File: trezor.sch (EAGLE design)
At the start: 38 parts, among them IC1 MCP1703CB, Q2 16MHz, U1 ATSHA204-TSU, U2 USB, U3 DISPLAY

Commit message: forgot to connect usb gnd/vcc
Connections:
- net +5V: now also U2.VBUS
- net GND: now also U2.GND
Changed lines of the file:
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@@
 <wire x1="99.06" y1="-20.32" x2="93.98" y2="-20.32" width="0.1524" layer="91"/>
 <wire x1="93.98" y1="-20.32" x2="93.98" y2="-25.4" width="0.1524" layer="91"/>
+<pinref part="U2" gate="G$1" pin="GND"/>
 </segment>
 </net>
@@
 <wire x1="109.22" y1="-22.86" x2="114.3" y2="-22.86" width="0.1524" layer="91"/>
 <wire x1="114.3" y1="-22.86" x2="114.3" y2="-20.32" width="0.1524" layer="91"/>
+<pinref part="U2" gate="G$1" pin="VBUS"/>
 </segment>
 </net>

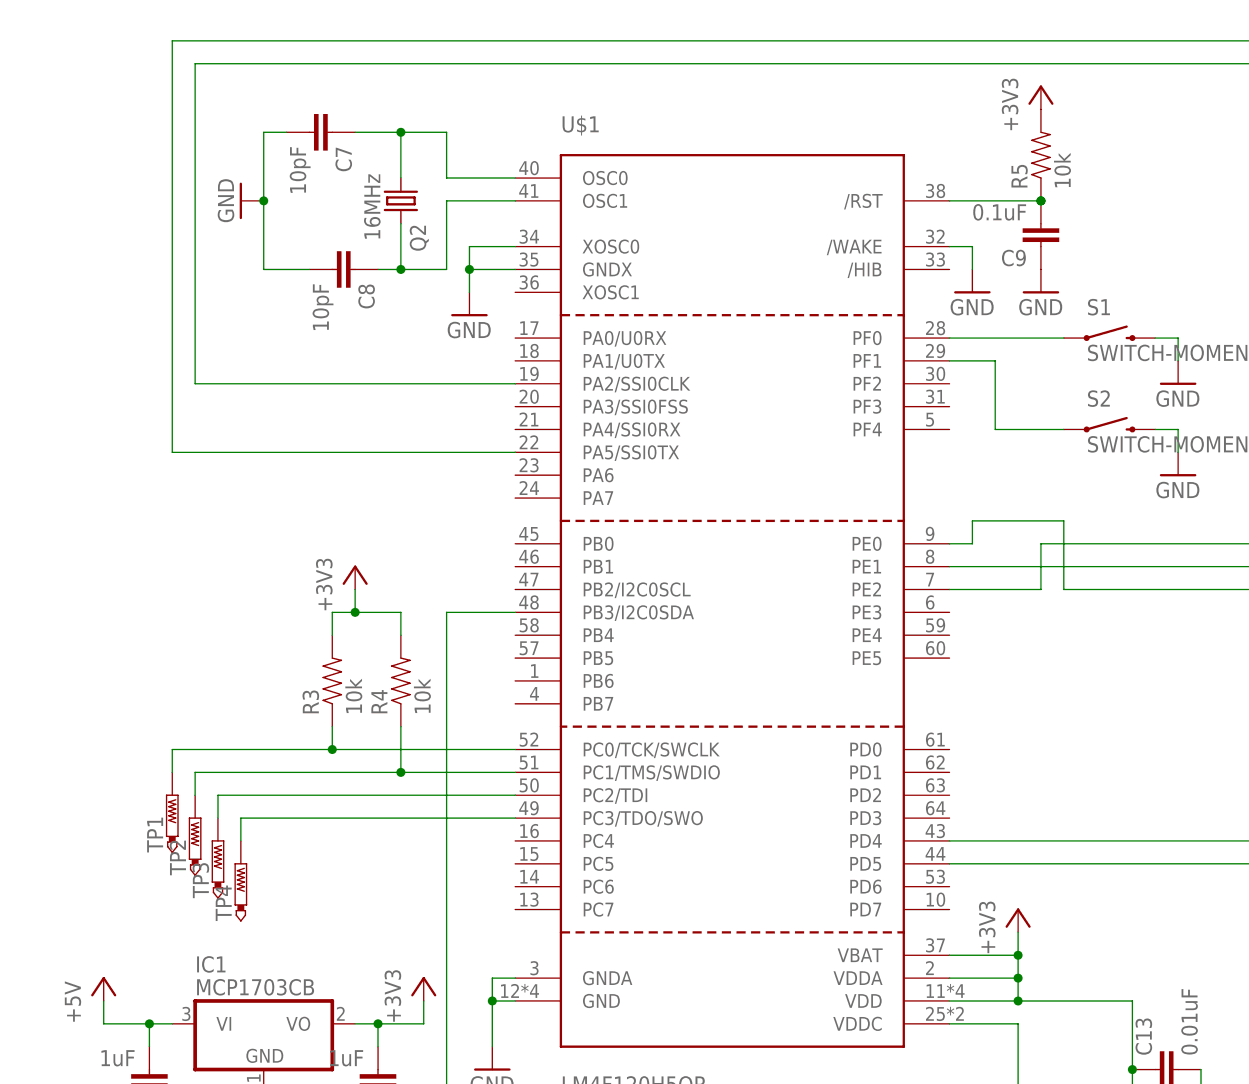
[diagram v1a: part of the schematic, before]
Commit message: wip
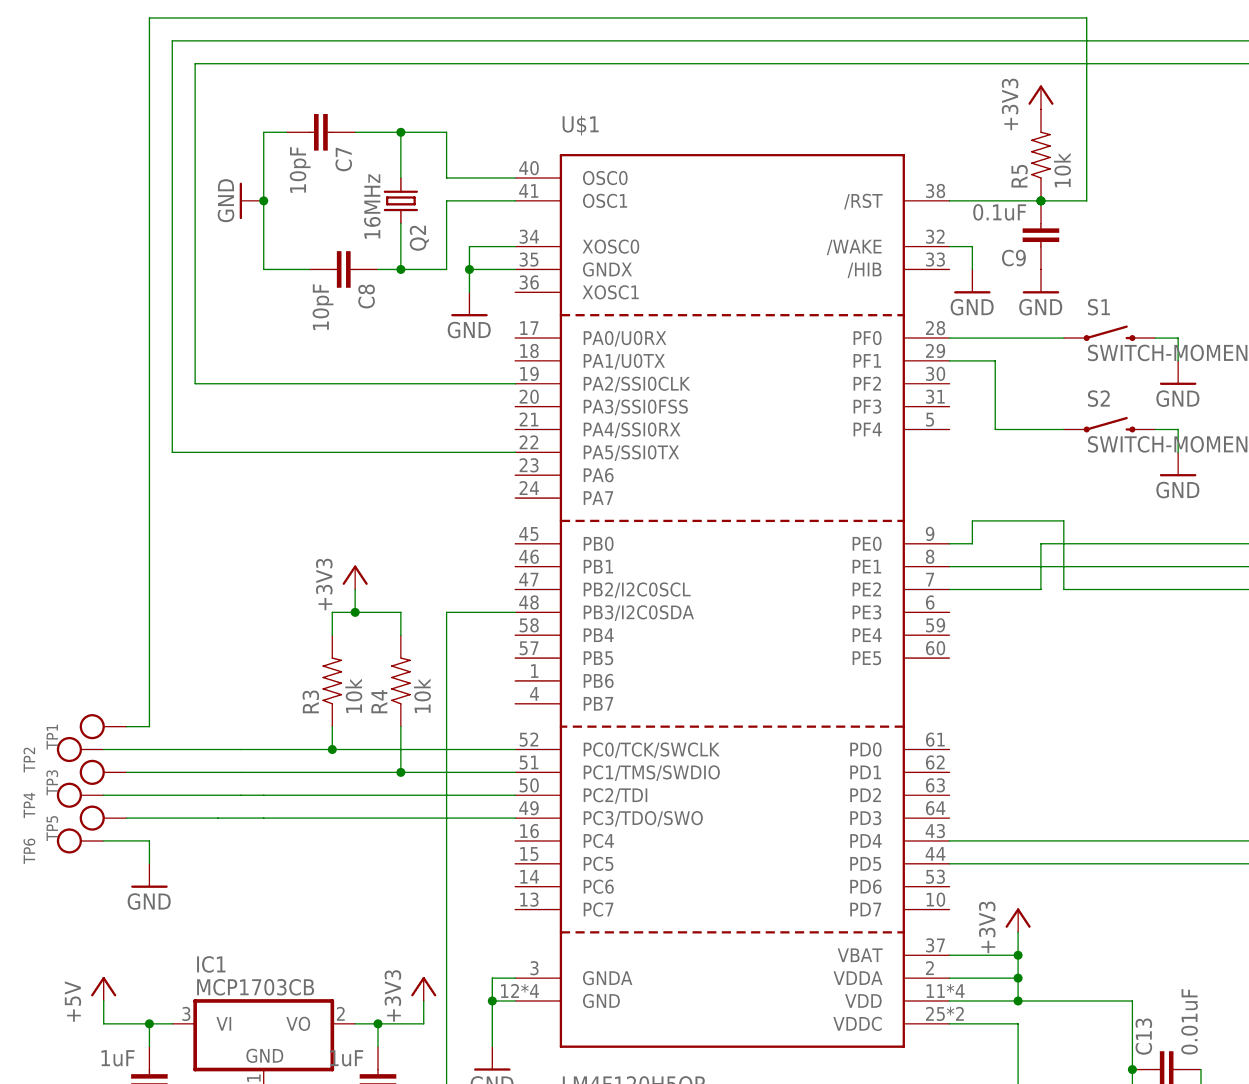
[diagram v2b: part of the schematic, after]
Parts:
- added TP5, TP6: (no value), microbuilder:TESTPOINTROUND0.5MM
- TP1, TP2, TP3, TP4: value PTR1TP10R -> (none); device testpad:PTR1TP10R -> microbuilder:TESTPOINTROUND0.5MM
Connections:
- net GND: now also TP6.P$1
- net N$16: now also TP3.P$1; no longer TP2.TP
- net N$17: now also TP2.P$1; no longer TP1.TP
- net N$19: now also TP4.P$1; no longer TP3.TP
- net N$20: now also TP5.P$1; no longer TP4.TP
- net N$21: now also TP1.P$1
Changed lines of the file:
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@@
 <part name="GND16" library="supply1" deviceset="GND" device=""/>
 <part name="+3V6" library="supply1" deviceset="+3V3" device=""/>
-<part name="TP1" library="testpad" deviceset="PTR1" device="TP10R"/>
-<part name="TP2" library="testpad" deviceset="PTR1" device="TP10R">
-<attribute name="TP_SIGNAL_NAME" value=""/>
-</part>
-<part name="TP3" library="testpad" deviceset="PTR1" device="TP10R">
-<attribute name="TP_SIGNAL_NAME" value=""/>
-</part>
-<part name="TP4" library="testpad" deviceset="PTR1" device="TP10R">
-<attribute name="TP_SIGNAL_NAME" value=""/>
-</part>
 <part name="IC1" library="linear" deviceset="MCP1703" device="CB"/>
 <part name="P+1" library="supply1" deviceset="+5V" device=""/>
 <part name="GND1" library="supply1" deviceset="GND" device=""/>
+<part name="GND17" library="supply1" deviceset="GND" device=""/>
+<part name="TP1" library="microbuilder" deviceset="TESTPOINT" device="ROUND0.5MM"/>
+<part name="TP2" library="microbuilder" deviceset="TESTPOINT" device="ROUND0.5MM"/>
+<part name="TP3" library="microbuilder" deviceset="TESTPOINT" device="ROUND0.5MM"/>
+<part name="TP4" library="microbuilder" deviceset="TESTPOINT" device="ROUND0.5MM"/>
+<part name="TP5" library="microbuilder" deviceset="TESTPOINT" device="ROUND0.5MM"/>
+<part name="TP6" library="microbuilder" deviceset="TESTPOINT" device="ROUND0.5MM"/>
 </parts>
 <sheets>
@@
 <instance part="GND16" gate="1" x="55.88" y="91.44"/>
 <instance part="+3V6" gate="G$1" x="55.88" y="114.3"/>
-<instance part="TP1" gate="G$1" x="-40.64" y="35.56"/>
-<instance part="TP2" gate="G$1" x="-38.1" y="33.02"/>
-<instance part="TP3" gate="G$1" x="-35.56" y="30.48"/>
-<instance part="TP4" gate="G$1" x="-33.02" y="27.94"/>
 <instance part="IC1" gate="G$1" x="-30.48" y="10.16"/>
 <instance part="P+1" gate="1" x="114.3" y="-17.78"/>
 <instance part="GND1" gate="1" x="93.98" y="-27.94"/>
+<instance part="GND17" gate="1" x="-43.18" y="25.4"/>
+<instance part="TP1" gate="G$1" x="-45.72" y="43.18" rot="R90"/>
+<instance part="TP2" gate="G$1" x="-48.26" y="40.64" rot="R90"/>
+<instance part="TP3" gate="G$1" x="-45.72" y="38.1" rot="R90"/>
+<instance part="TP4" gate="G$1" x="-48.26" y="35.56" rot="R90"/>
+<instance part="TP5" gate="G$1" x="-45.72" y="33.02" rot="R90"/>
+<instance part="TP6" gate="G$1" x="-48.26" y="30.48" rot="R90"/>
 </instances>
 <busses>
@@
 <pinref part="U2" gate="G$1" pin="GND"/>
 </segment>
+<segment>
+<pinref part="GND17" gate="1" pin="GND"/>
+<wire x1="-43.18" y1="27.94" x2="-43.18" y2="30.48" width="0.1524" layer="91"/>
+<wire x1="-43.18" y1="30.48" x2="-48.26" y2="30.48" width="0.1524" layer="91"/>
+<pinref part="TP6" gate="G$1" pin="P$1"/>
+</segment>
 </net>
 <net name="N$8" class="0">
@@
 <pinref part="R3" gate="G$1" pin="1"/>
 <wire x1="-22.86" y1="43.18" x2="-22.86" y2="40.64" width="0.1524" layer="91"/>
+<wire x1="-22.86" y1="40.64" x2="-33.02" y2="40.64" width="0.1524" layer="91"/>
 <junction x="-22.86" y="40.64"/>
-<pinref part="TP1" gate="G$1" pin="TP"/>
-<wire x1="-22.86" y1="40.64" x2="-40.64" y2="40.64" width="0.1524" layer="91"/>
-<wire x1="-40.64" y1="40.64" x2="-40.64" y2="38.1" width="0.1524" layer="91"/>
+<wire x1="-33.02" y1="40.64" x2="-48.26" y2="40.64" width="0.1524" layer="91"/>
+<pinref part="TP2" gate="G$1" pin="P$1"/>
 </segment>
 </net>
@@
 <pinref part="R4" gate="G$1" pin="1"/>
 <wire x1="-15.24" y1="43.18" x2="-15.24" y2="38.1" width="0.1524" layer="91"/>
+<wire x1="-15.24" y1="38.1" x2="-33.02" y2="38.1" width="0.1524" layer="91"/>
 <junction x="-15.24" y="38.1"/>
-<pinref part="TP2" gate="G$1" pin="TP"/>
-<wire x1="-15.24" y1="38.1" x2="-38.1" y2="38.1" width="0.1524" layer="91"/>
-<wire x1="-38.1" y1="38.1" x2="-38.1" y2="35.56" width="0.1524" layer="91"/>
+<wire x1="-33.02" y1="38.1" x2="-45.72" y2="38.1" width="0.1524" layer="91"/>
+<pinref part="TP3" gate="G$1" pin="P$1"/>
 </segment>
 </net>
@@
 <segment>
 <pinref part="U$1" gate="G$1" pin="PC2/TDI"/>
-<wire x1="-2.54" y1="35.56" x2="-35.56" y2="35.56" width="0.1524" layer="91"/>
-<pinref part="TP3" gate="G$1" pin="TP"/>
-<wire x1="-35.56" y1="35.56" x2="-35.56" y2="33.02" width="0.1524" layer="91"/>
+<wire x1="-2.54" y1="35.56" x2="-30.48" y2="35.56" width="0.1524" layer="91"/>
+<wire x1="-30.48" y1="35.56" x2="-33.02" y2="35.56" width="0.1524" layer="91"/>
+<wire x1="-33.02" y1="35.56" x2="-48.26" y2="35.56" width="0.1524" layer="91"/>
+<pinref part="TP4" gate="G$1" pin="P$1"/>
 </segment>
 </net>
@@
 <segment>
 <pinref part="U$1" gate="G$1" pin="PC3/TDO/SWO"/>
-<wire x1="-2.54" y1="33.02" x2="-33.02" y2="33.02" width="0.1524" layer="91"/>
-<wire x1="-33.02" y1="33.02" x2="-33.02" y2="30.48" width="0.1524" layer="91"/>
-<pinref part="TP4" gate="G$1" pin="TP"/>
+<wire x1="-2.54" y1="33.02" x2="-30.48" y2="33.02" width="0.1524" layer="91"/>
+<wire x1="-30.48" y1="33.02" x2="-35.56" y2="33.02" width="0.1524" layer="91"/>
+<wire x1="-35.56" y1="33.02" x2="-45.72" y2="33.02" width="0.1524" layer="91"/>
+<pinref part="TP5" gate="G$1" pin="P$1"/>
 </segment>
 </net>
@@
 <junction x="55.88" y="101.6"/>
 <junction x="55.88" y="101.6"/>
-</segment>
-</net>
+<wire x1="55.88" y1="101.6" x2="60.96" y2="101.6" width="0.1524" layer="91"/>
+<wire x1="60.96" y1="101.6" x2="60.96" y2="121.92" width="0.1524" layer="91"/>
+<wire x1="60.96" y1="121.92" x2="-43.18" y2="121.92" width="0.1524" layer="91"/>
+<wire x1="-43.18" y1="121.92" x2="-43.18" y2="43.18" width="0.1524" layer="91"/>
+<wire x1="-43.18" y1="43.18" x2="-45.72" y2="43.18" width="0.1524" layer="91"/>
+<pinref part="TP1" gate="G$1" pin="P$1"/>
+</segment>
+</net>

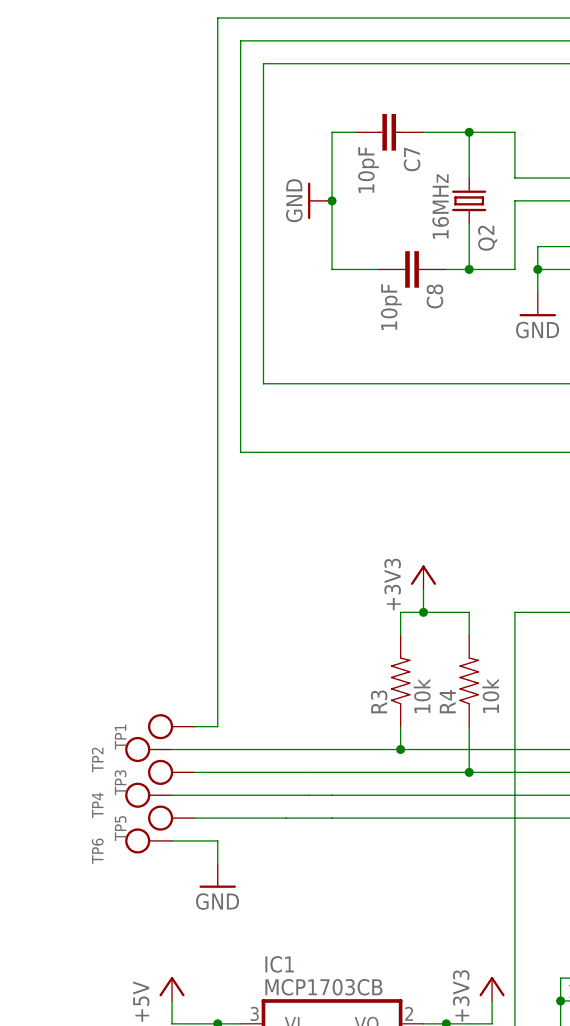
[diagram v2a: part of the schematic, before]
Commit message: wip
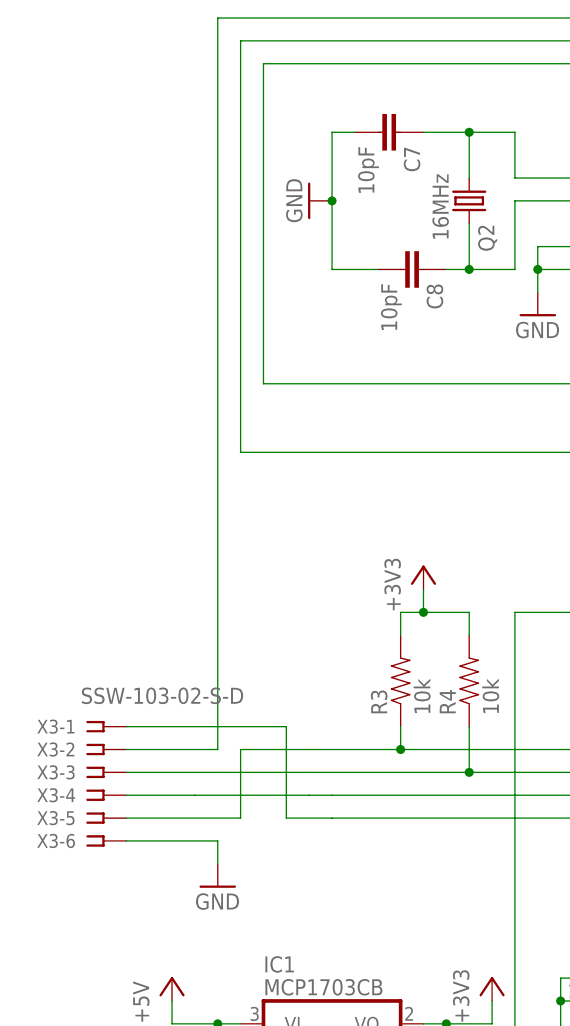
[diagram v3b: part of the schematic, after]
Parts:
- removed TP1, TP2, TP3, TP4, TP5, TP6: (no value), microbuilder:TESTPOINTROUND0.5MM
- added X3: SSW-103-02-S-D, con-samtec:SSW-103-02-S-D
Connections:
- net GND: now also X3-6.1; no longer TP6.P$1
- net N$16: now also X3-3.1; no longer TP3.P$1
- net N$17: now also X3-5.1; no longer TP2.P$1
- net N$19: now also X3-4.1; no longer TP4.P$1
- net N$20: now also X3-1.1; no longer TP5.P$1
- net N$21: now also X3-2.1; no longer TP1.P$1
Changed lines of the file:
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@@
 <part name="GND1" library="supply1" deviceset="GND" device=""/>
 <part name="GND17" library="supply1" deviceset="GND" device=""/>
-<part name="TP1" library="microbuilder" deviceset="TESTPOINT" device="ROUND0.5MM"/>
-<part name="TP2" library="microbuilder" deviceset="TESTPOINT" device="ROUND0.5MM"/>
-<part name="TP3" library="microbuilder" deviceset="TESTPOINT" device="ROUND0.5MM"/>
-<part name="TP4" library="microbuilder" deviceset="TESTPOINT" device="ROUND0.5MM"/>
-<part name="TP5" library="microbuilder" deviceset="TESTPOINT" device="ROUND0.5MM"/>
-<part name="TP6" library="microbuilder" deviceset="TESTPOINT" device="ROUND0.5MM"/>
+<part name="X3" library="con-samtec" deviceset="SSW-103-02-S-D" device=""/>
 </parts>
 <sheets>
@@
 <instance part="GND1" gate="1" x="93.98" y="-27.94"/>
 <instance part="GND17" gate="1" x="-43.18" y="25.4"/>
-<instance part="TP1" gate="G$1" x="-45.72" y="43.18" rot="R90"/>
-<instance part="TP2" gate="G$1" x="-48.26" y="40.64" rot="R90"/>
-<instance part="TP3" gate="G$1" x="-45.72" y="38.1" rot="R90"/>
-<instance part="TP4" gate="G$1" x="-48.26" y="35.56" rot="R90"/>
-<instance part="TP5" gate="G$1" x="-45.72" y="33.02" rot="R90"/>
-<instance part="TP6" gate="G$1" x="-48.26" y="30.48" rot="R90"/>
+<instance part="X3" gate="-1" x="-55.88" y="43.18"/>
+<instance part="X3" gate="-2" x="-55.88" y="40.64"/>
+<instance part="X3" gate="-3" x="-55.88" y="38.1"/>
+<instance part="X3" gate="-4" x="-55.88" y="35.56"/>
+<instance part="X3" gate="-5" x="-55.88" y="33.02"/>
+<instance part="X3" gate="-6" x="-55.88" y="30.48"/>
 </instances>
 <busses>
@@
 </segment>
 <segment>
+<pinref part="X3" gate="-6" pin="1"/>
 <pinref part="GND17" gate="1" pin="GND"/>
-<wire x1="-43.18" y1="27.94" x2="-43.18" y2="30.48" width="0.1524" layer="91"/>
-<wire x1="-43.18" y1="30.48" x2="-48.26" y2="30.48" width="0.1524" layer="91"/>
-<pinref part="TP6" gate="G$1" pin="P$1"/>
+<wire x1="-53.34" y1="30.48" x2="-43.18" y2="30.48" width="0.1524" layer="91"/>
+<wire x1="-43.18" y1="30.48" x2="-43.18" y2="27.94" width="0.1524" layer="91"/>
 </segment>
 </net>
@@
 <wire x1="-22.86" y1="40.64" x2="-33.02" y2="40.64" width="0.1524" layer="91"/>
 <junction x="-22.86" y="40.64"/>
-<wire x1="-33.02" y1="40.64" x2="-48.26" y2="40.64" width="0.1524" layer="91"/>
-<pinref part="TP2" gate="G$1" pin="P$1"/>
+<wire x1="-33.02" y1="40.64" x2="-40.64" y2="40.64" width="0.1524" layer="91"/>
+<wire x1="-40.64" y1="40.64" x2="-40.64" y2="33.02" width="0.1524" layer="91"/>
+<pinref part="X3" gate="-5" pin="1"/>
+<wire x1="-40.64" y1="33.02" x2="-53.34" y2="33.02" width="0.1524" layer="91"/>
 </segment>
 </net>
@@
 <wire x1="-15.24" y1="38.1" x2="-33.02" y2="38.1" width="0.1524" layer="91"/>
 <junction x="-15.24" y="38.1"/>
-<wire x1="-33.02" y1="38.1" x2="-45.72" y2="38.1" width="0.1524" layer="91"/>
-<pinref part="TP3" gate="G$1" pin="P$1"/>
+<wire x1="-33.02" y1="38.1" x2="-43.18" y2="38.1" width="0.1524" layer="91"/>
+<pinref part="X3" gate="-3" pin="1"/>
+<wire x1="-43.18" y1="38.1" x2="-53.34" y2="38.1" width="0.1524" layer="91"/>
 </segment>
 </net>
@@
 <wire x1="-2.54" y1="35.56" x2="-30.48" y2="35.56" width="0.1524" layer="91"/>
 <wire x1="-30.48" y1="35.56" x2="-33.02" y2="35.56" width="0.1524" layer="91"/>
-<wire x1="-33.02" y1="35.56" x2="-48.26" y2="35.56" width="0.1524" layer="91"/>
-<pinref part="TP4" gate="G$1" pin="P$1"/>
+<wire x1="-33.02" y1="35.56" x2="-45.72" y2="35.56" width="0.1524" layer="91"/>
+<pinref part="X3" gate="-4" pin="1"/>
+<wire x1="-45.72" y1="35.56" x2="-53.34" y2="35.56" width="0.1524" layer="91"/>
 </segment>
 </net>
@@
 <wire x1="-2.54" y1="33.02" x2="-30.48" y2="33.02" width="0.1524" layer="91"/>
 <wire x1="-30.48" y1="33.02" x2="-35.56" y2="33.02" width="0.1524" layer="91"/>
-<wire x1="-35.56" y1="33.02" x2="-45.72" y2="33.02" width="0.1524" layer="91"/>
-<pinref part="TP5" gate="G$1" pin="P$1"/>
+<wire x1="-35.56" y1="33.02" x2="-35.56" y2="43.18" width="0.1524" layer="91"/>
+<pinref part="X3" gate="-1" pin="1"/>
+<wire x1="-35.56" y1="43.18" x2="-53.34" y2="43.18" width="0.1524" layer="91"/>
 </segment>
 </net>
@@
 <wire x1="60.96" y1="101.6" x2="60.96" y2="121.92" width="0.1524" layer="91"/>
 <wire x1="60.96" y1="121.92" x2="-43.18" y2="121.92" width="0.1524" layer="91"/>
-<wire x1="-43.18" y1="121.92" x2="-43.18" y2="43.18" width="0.1524" layer="91"/>
-<wire x1="-43.18" y1="43.18" x2="-45.72" y2="43.18" width="0.1524" layer="91"/>
-<pinref part="TP1" gate="G$1" pin="P$1"/>
-</segment>
-</net>
+<wire x1="-43.18" y1="121.92" x2="-43.18" y2="40.64" width="0.1524" layer="91"/>
+<pinref part="X3" gate="-2" pin="1"/>
+<wire x1="-43.18" y1="40.64" x2="-53.34" y2="40.64" width="0.1524" layer="91"/>
+</segment>
+</net>

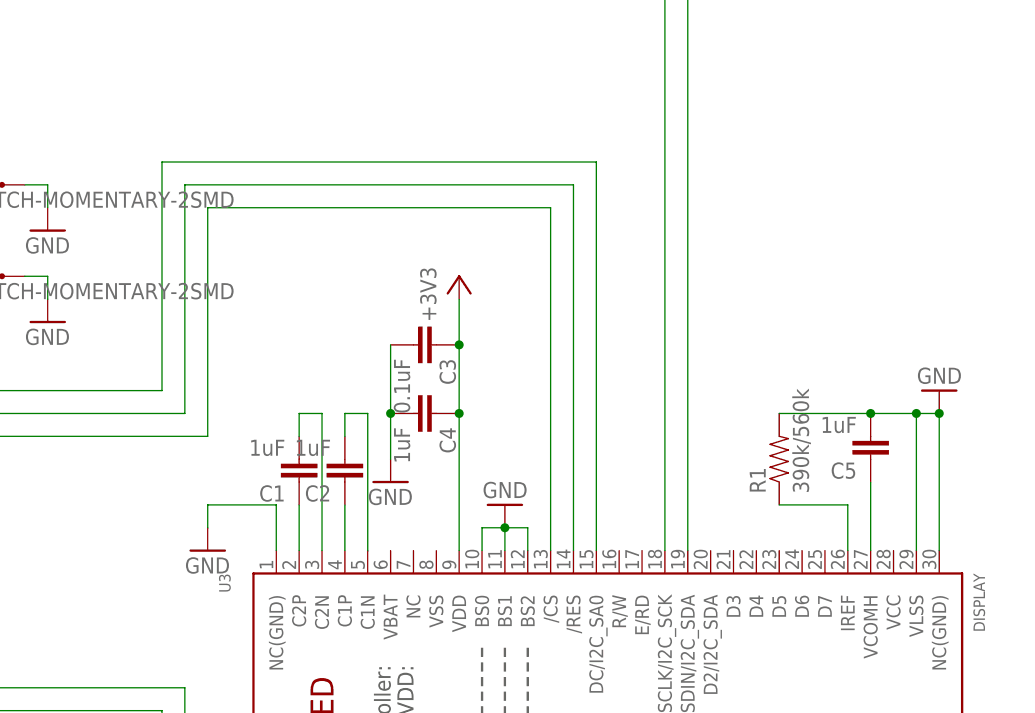
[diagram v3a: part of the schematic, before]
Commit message: wip
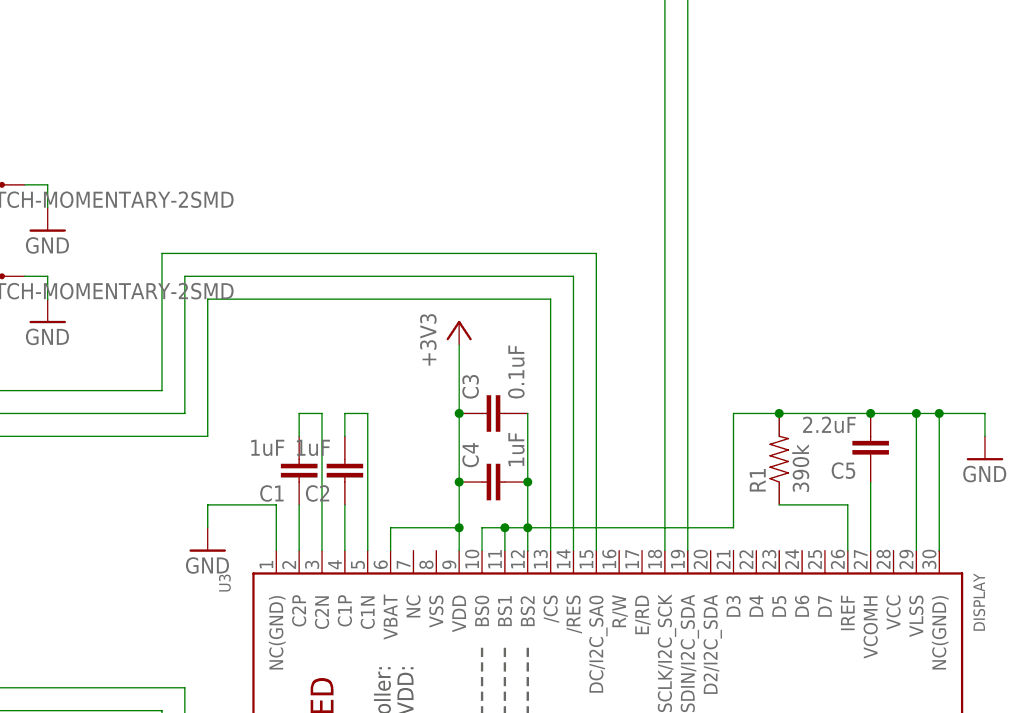
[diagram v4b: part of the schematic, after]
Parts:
- C5: value 1uF -> 2.2uF
- R1: value 390k/560k -> 390k
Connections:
- net +3V3: now also U3.VBAT
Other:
- moved on the sheet: C3, C4
